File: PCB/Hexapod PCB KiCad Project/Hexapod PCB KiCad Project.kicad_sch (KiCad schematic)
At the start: 33 parts, among them T1 Battery, T2 Switch, U1 DEV-16771, U3 NRF24L01_Breakout, U4 Gyro MPU6050, U5 Buck Converter 5V MP1584EN

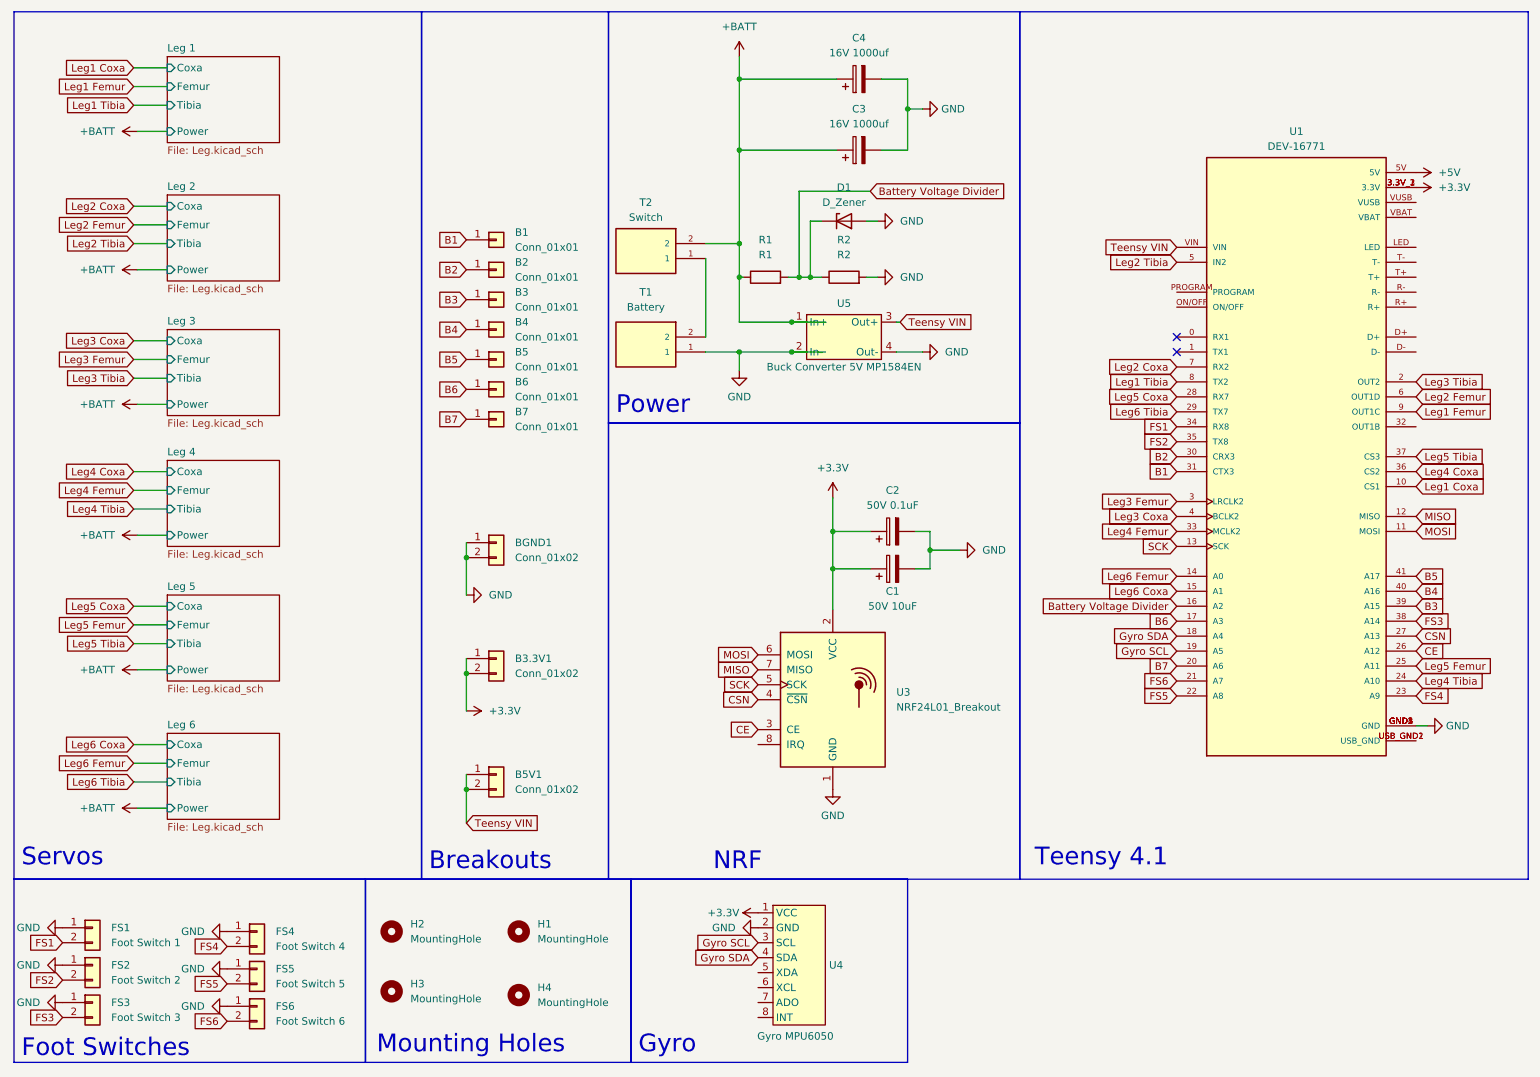
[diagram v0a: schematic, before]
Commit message: breakout updates
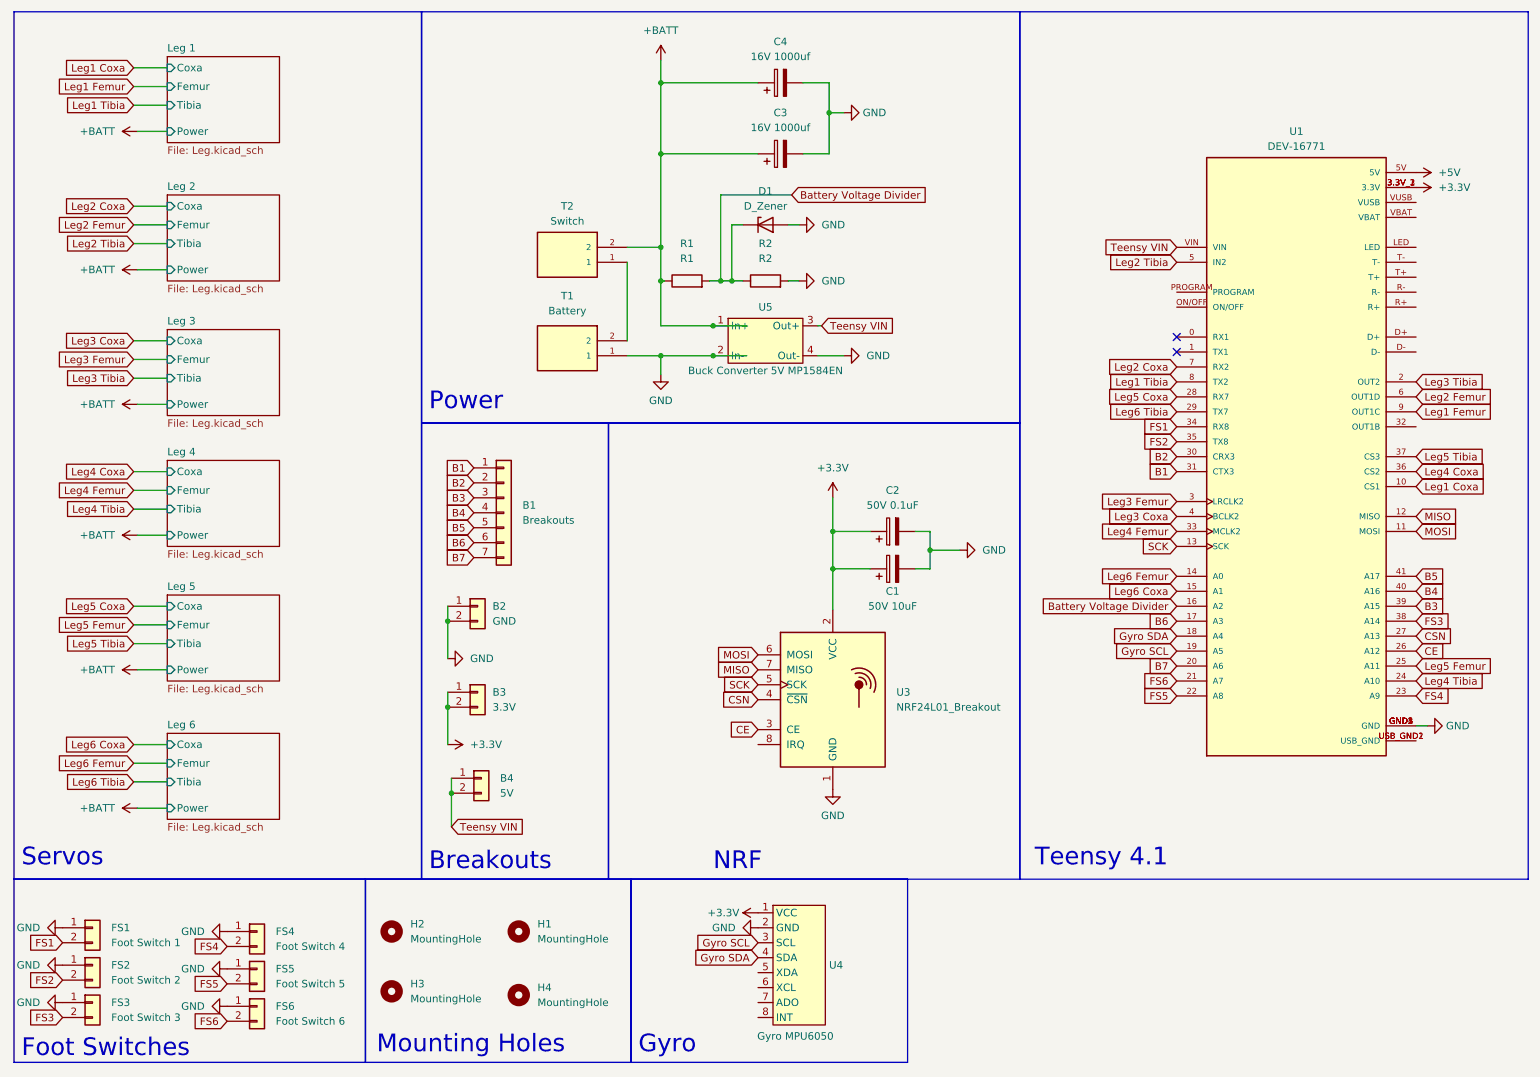
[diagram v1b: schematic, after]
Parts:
- removed B2, B3, B4, B5, B6, B7: Conn_01x01, Connector_PinHeader_2.54mm:PinHeader_1x01_P2.54mm_Vertical, symbol Connector_Generic:Conn_01x01
- B1: value Conn_01x01 -> Breakouts; footprint Connector_PinHeader_2.54mm:PinHeader_1x01_P2.54mm_Vertical -> Connector_PinSocket_2.54mm:PinSocket_1x07_P2.54mm_Vertical; symbol Connector_Generic:Conn_01x01 -> Connector_Generic:Conn_01x07
- B2: renamed from BGND1; value Conn_01x02 -> GND; footprint Connector_PinHeader_2.54mm:PinHeader_1x02_P2.54mm_Vertical -> Connector_PinSocket_2.54mm:PinSocket_1x02_P2.54mm_Vertical
- B3: renamed from B3.3V1; value Conn_01x02 -> 3.3V; footprint Connector_PinHeader_2.54mm:PinHeader_1x02_P2.54mm_Vertical -> Connector_PinSocket_2.54mm:PinSocket_1x02_P2.54mm_Vertical
- B4: renamed from B5V1; value Conn_01x02 -> 5V; footprint Connector_PinHeader_2.54mm:PinHeader_1x02_P2.54mm_Vertical -> Connector_PinSocket_2.54mm:PinSocket_1x02_P2.54mm_Vertical
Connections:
- net B2: now also B1.2 (Pin_2)
- net B3: now also B1.3 (Pin_3)
- net B4: now also B1.4 (Pin_4)
- net B5: now also B1.5 (Pin_5)
- net B6: now also B1.6 (Pin_6)
- net B7: now also B1.7 (Pin_7)
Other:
- moved on the sheet: B2, B3, B4, C3, C4, D1, R1, R2, T1, T2, U5
